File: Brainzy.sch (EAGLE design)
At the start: 74 parts, among them J7 5.5x2.1mm Barrel, M1 WIRELESS-NRF24L01, Q1 BSS138, Q2 BSS138, Q3 BSS138, T1 BSS84, T2 BSS84, T3 BSS84, T4 S12323DS, U1 L293DD, U2 L293DD, U3 HC_05, U4 GY-521MPU6050

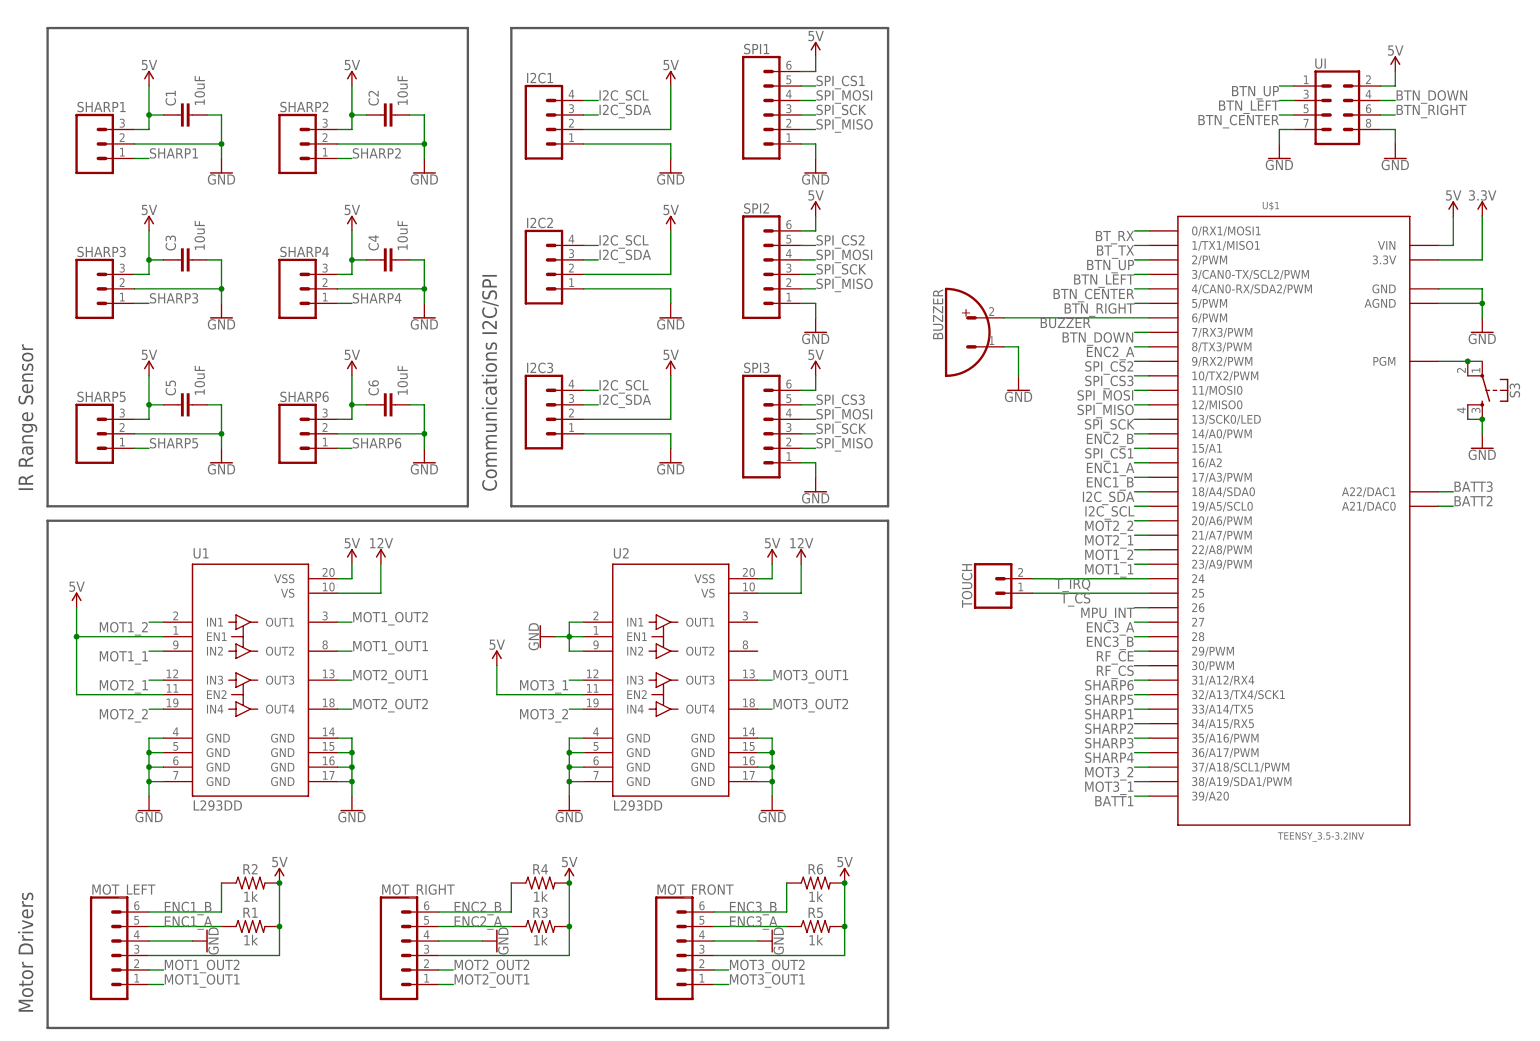
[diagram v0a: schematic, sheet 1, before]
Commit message: Upload Brainzy v2.1
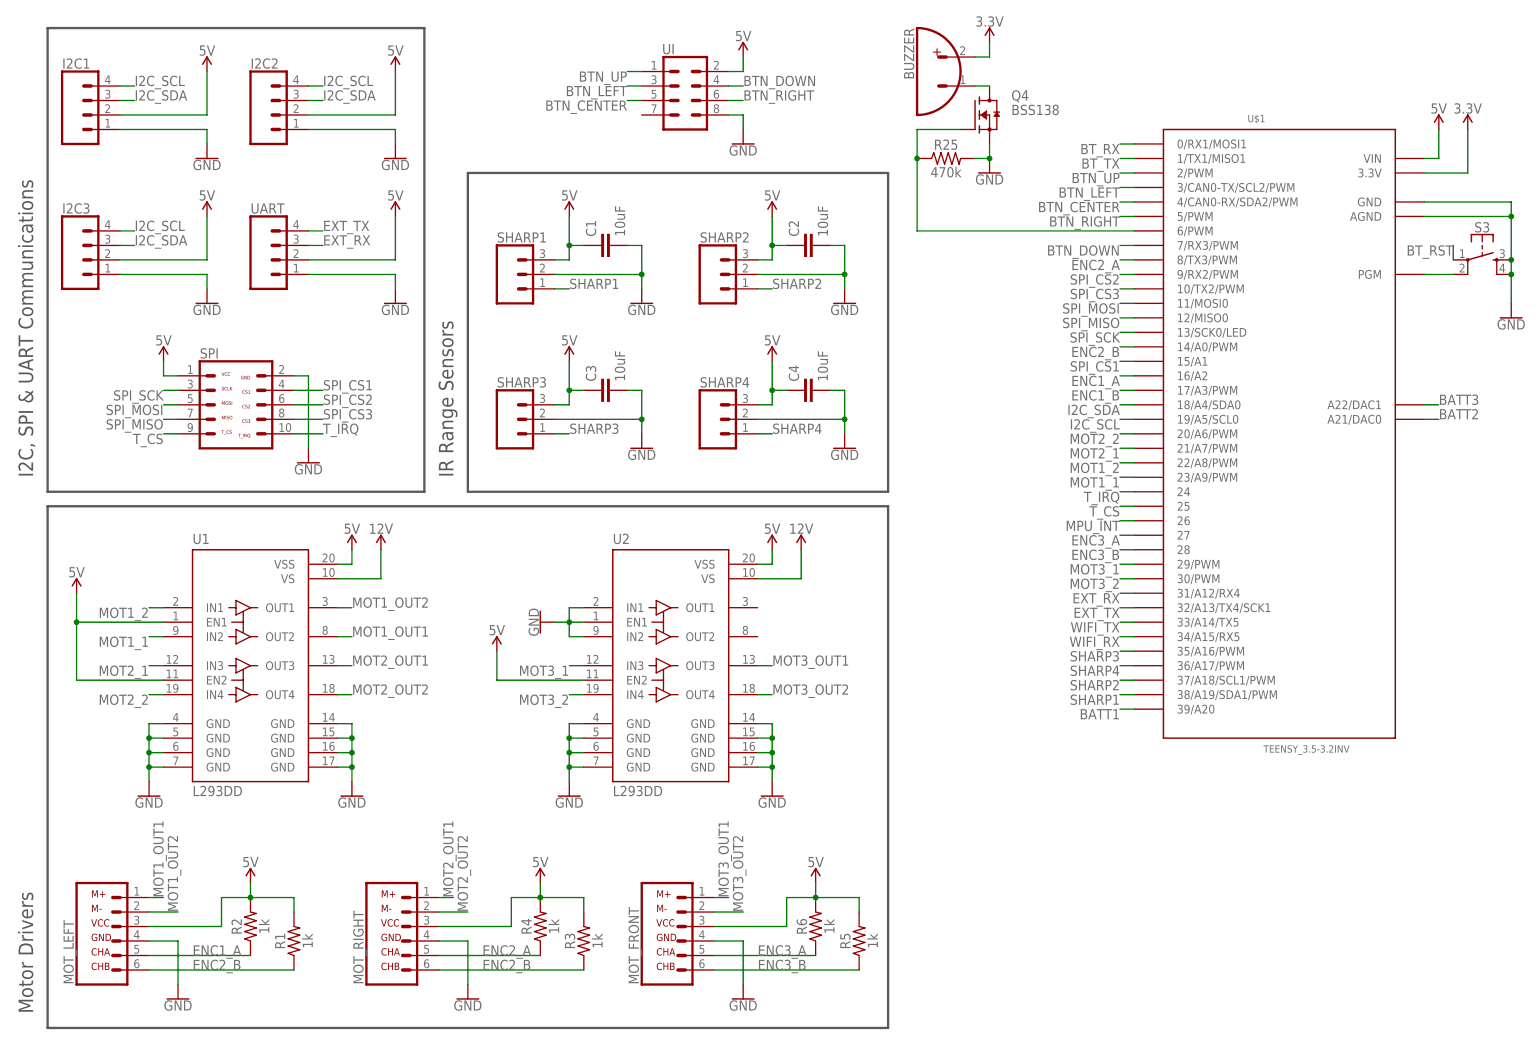
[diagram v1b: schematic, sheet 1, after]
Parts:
- removed C5, C6: 10uF, SparkFun-Capacitors:10UF-1206-6.3V-20%
- removed C7: 100nF, SparkFun-Capacitors:10UF-1206-6.3V-20%
- removed M1: WIRELESS-NRF24L01, MrRobotics-Modules:WIRELESS-NRF24L01
- removed SHARP5, SHARP6: (no value), SparkFun-Connectors:CONN_03
- removed SPI1, SPI2, SPI3: JST-XH-06-PIN-ROUND-PAD, MrRobotics-Connectors:JST-XH-06-PIN-ROUND-PAD
- removed TOUCH: JST-XH-02-PIN-ROUND-PAD, MrRobotics-Connectors:JST-XH-02-PIN-ROUND-PAD
- added EXT_BT: (no value), SparkFun-Connectors:CONN_041X04_NO_SILK
- added Q4: BSS138, MrRobotics-Transistors:BSS138
- added R22: 10k, SparkFun-Resistors:10OHM-1206-1/4W-1%
- added R23, R25: 470k, SparkFun-Resistors:10OHM-1206-1/4W-1%
- added R24: 150k, SparkFun-Resistors:10OHM-1206-1/4W-1%
- added SPI: (no value), MrRobotics-Connectors:CONN_05X2_EXTSHD_LOCK
- added U$6: WIRELESS-WIFI-ESP-01, MrRobotics-Modules:WIRELESS-WIFI-ESP-01
- added UART: (no value), SparkFun-Connectors:CONN_04
- BATT: value JST-XH-04-PIN-ROUND-PAD -> BATTERY-CONNECTOR-LONG-PAD; device MrRobotics-Connectors:JST-XH-04-PIN-ROUND-PAD -> MrRobotics-Connectors:BATTERY-CONNECTOR-LONG-PAD
- MOT_FRONT, MOT_LEFT, MOT_RIGHT: value JST-XH-06-PIN-ROUND-PAD -> (none); device MrRobotics-Connectors:JST-XH-06-PIN-ROUND-PAD -> MrRobotics-Connectors:DC-MOTOR-CONNECTOR
- T4: value S12323DS -> SI2323DS; device MrRobotics-Transistors:S12323DS -> MrRobotics-Transistors:SI2323DS
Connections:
- removed net BUZZER: BUZZER.1, U$1.6/PWM
- removed net RF_CE: M1.CE, U$1.29/PWM
- removed net RF_CS: M1.CSN, U$1.30/PWM
- removed net SHARP5: SHARP5.1, U$1.32/A13/TX4/SCK1
- removed net SHARP6: SHARP6.1, U$1.31/A12/RX4
- new net BT_RST: S3.1, U3.RST
- new net EXT_RX: U$1.31/A12/RX4, UART.3
- new net EXT_TX: U$1.32/A13/TX4/SCK1, UART.4
- new net N$19: R23.2, T1.D
- new net N$20: BUZZER.3, Q4.D
- new net N$3: R22.1, U$6.CH_PD
- new net N$8: Q4.G, R25.1, U$1.6/PWM
- new net WIFI_RX: U$1.34/A15/RX5, U$6.UTXD
- new net WIFI_TX: U$1.33/A14/TX5, U$6.URXD
- net 3.3V: now also BUZZER.1, R22.2, U$6.VCC; no longer C7.2, M1.VCC
- net 5V: now also EXT_BT.1, MOT_FRONT.3-VCC, MOT_LEFT.3-VCC, MOT_RIGHT.3-VCC, SPI.1-VCC, UART.2; no longer C5.1, C6.1, MOT_FRONT.3, MOT_LEFT.3, MOT_RIGHT.3, SHARP5.3, SHARP6.3, SPI1.6, SPI2.6, SPI3.6
- net BATT1: now also R23.1, R24.2; no longer T1.D
- net BT_RX: now also EXT_BT.3
- net BT_TX: now also EXT_BT.4
- net ENC1_A: now also MOT_LEFT.5-CHA, R2.1; no longer MOT_LEFT.5, R1.1
- net ENC1_B: no longer MOT_LEFT.6, R2.1
- net ENC2_A: now also MOT_RIGHT.5-CHA, R4.1; no longer MOT_RIGHT.5, R3.1
- net ENC2_B: now also MOT_LEFT.6-CHB, MOT_RIGHT.6-CHB, R1.1, R3.1; no longer MOT_RIGHT.6, R4.1
- net ENC3_A: now also MOT_FRONT.5-CHA, R6.1; no longer MOT_FRONT.5, R5.1
- net ENC3_B: now also MOT_FRONT.6-CHB, R5.1; no longer MOT_FRONT.6, R6.1
- net GND: now also BATT.1-GND, EXT_BT.2, MOT_FRONT.4-GND, MOT_LEFT.4-GND, MOT_RIGHT.4-GND, Q4.S, R24.1, R25.2, SPI.2-GND, U$6.GND, UART.1; no longer BATT.1, BUZZER.3, C5.2, C6.2, C7.1, M1.GND, MOT_FRONT.4, MOT_LEFT.4, MOT_RIGHT.4, SHARP5.2, SHARP6.2, SPI1.1, SPI2.1, SPI3.1, UI.7
- net MOT1_OUT1: now also MOT_LEFT.1-M-; no longer MOT_LEFT.1
- net MOT1_OUT2: now also MOT_LEFT.2-M+; no longer MOT_LEFT.2
- net MOT2_OUT1: now also MOT_RIGHT.1-M-; no longer MOT_RIGHT.1
- net MOT2_OUT2: now also MOT_RIGHT.2-M+; no longer MOT_RIGHT.2
- net MOT3_1: now also U$1.29/PWM; no longer U$1.38/A19/SDA1/PWM
- net MOT3_2: now also U$1.30/PWM; no longer U$1.37/A18/SCL1/PWM
- net MOT3_OUT1: now also MOT_FRONT.1-M-; no longer MOT_FRONT.1
- net MOT3_OUT2: now also MOT_FRONT.2-M+; no longer MOT_FRONT.2
- net N$12: no longer S3.1
- net S1: now also BATT.2-S1; no longer BATT.2
- net S2: now also BATT.3-S2; no longer BATT.3
- net S3: now also BATT.4-S3; no longer BATT.4
- net SHARP1: now also U$1.38/A19/SDA1/PWM; no longer U$1.33/A14/TX5
- net SHARP2: now also U$1.37/A18/SCL1/PWM; no longer U$1.34/A15/RX5
- net SPI_CS1: now also SPI.4-CS1; no longer SPI1.5
- net SPI_CS2: now also SPI.6-CS2; no longer SPI2.5
- net SPI_CS3: now also SPI.8-CS3; no longer SPI3.5
- net SPI_MISO: now also SPI.7-MISO; no longer M1.MISO, SPI1.2, SPI2.2, SPI3.2
- net SPI_MOSI: now also SPI.5-MOSI; no longer M1.MOSI, SPI1.4, SPI2.4, SPI3.4
- net SPI_SCK: now also SPI.3-SCLK; no longer M1.SCK, SPI1.3, SPI2.3, SPI3.3
- net T_CS: now also SPI.9-T_CS; no longer TOUCH.1
- net T_IRQ: now also SPI.10-T_IRQ; no longer TOUCH.2
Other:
- note added: "Extension for HC-05/06 breakout board"
- note added: "I2C, SPI & UART Communications"
- note added: "IR Range Sensors"
- note added: "JP1 selects between I2C addresses 0x68 and 0x69"
- note added: "Wifi & Bluetooth Communications"
- note removed: "Communications I2C/SPI"
- note removed: "IR Range Sensor"
- note removed: "JP1 selects between I2C address 0x68 and 0x69"
- note removed: "Radio Communications"
- moved on the sheet: BUZZER, C1, C2, C3, C4, D1, D2, I2C1, I2C2, I2C3, J7, Q1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
